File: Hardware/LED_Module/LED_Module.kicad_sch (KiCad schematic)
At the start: 4 parts

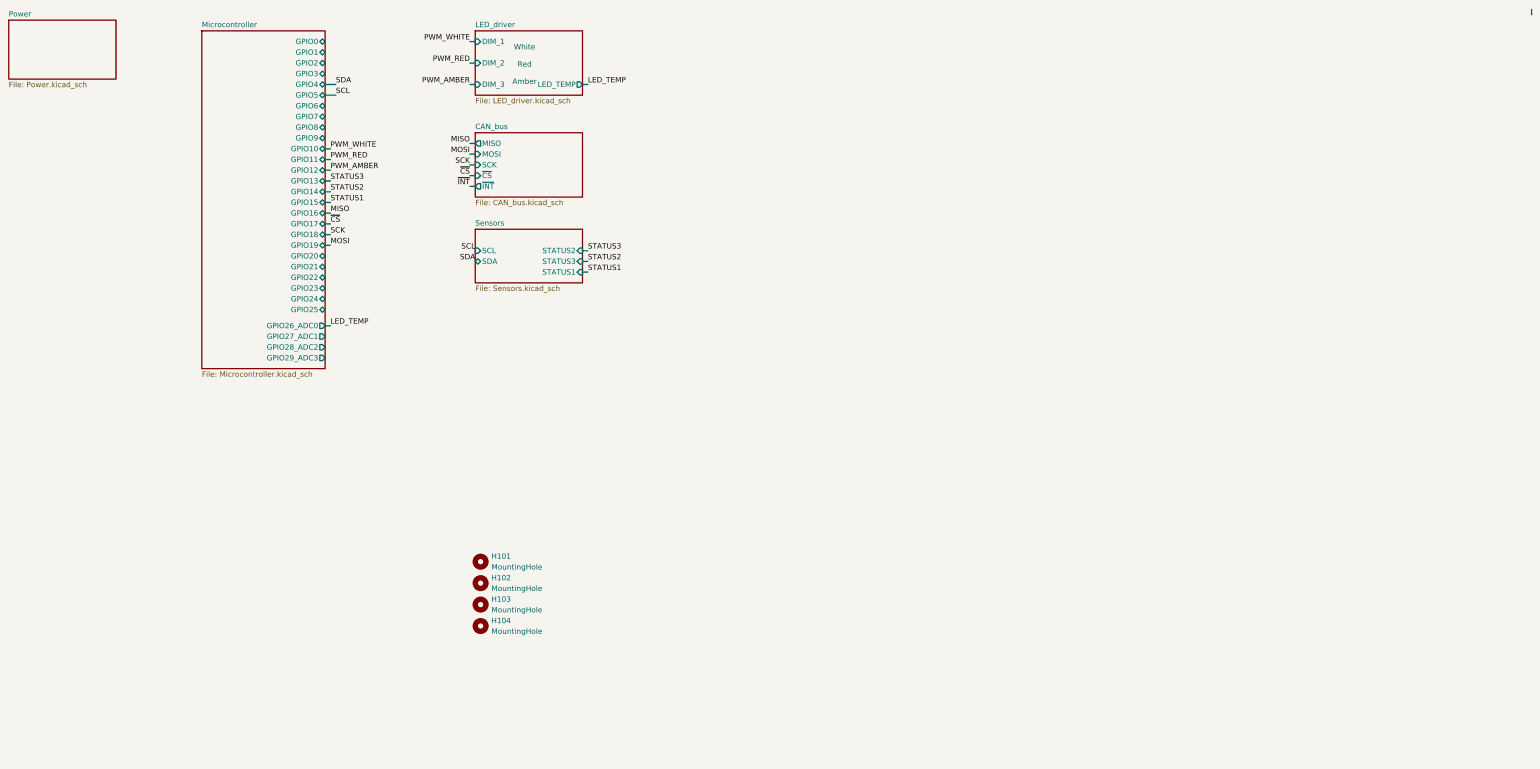
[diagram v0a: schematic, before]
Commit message: final fixes (hopefully) (GONE WRONG?!) (real)
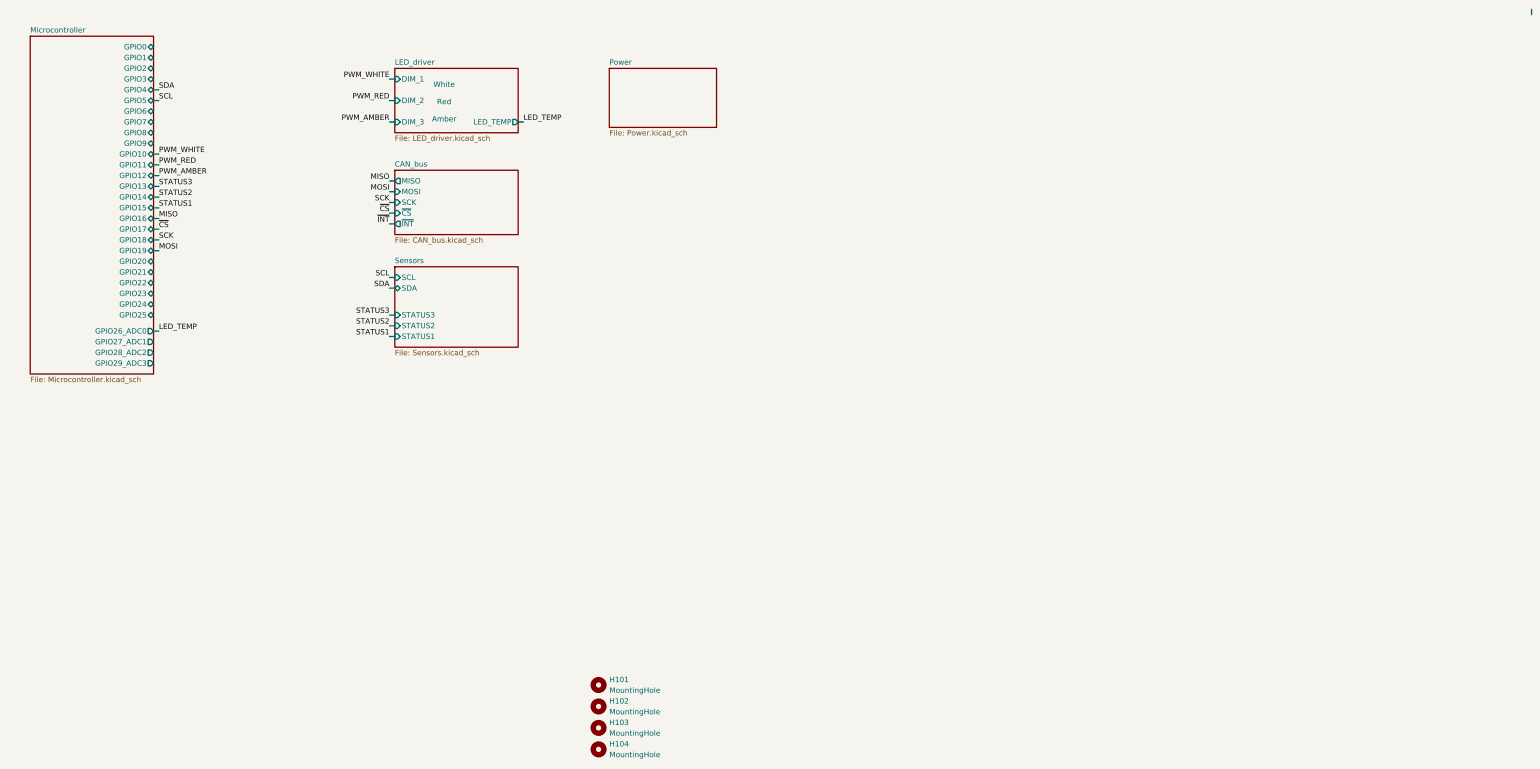
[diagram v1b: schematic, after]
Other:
- title: (none) -> Illumination system LED Module - overview
- moved on the sheet: H101, H102, H103, H104
